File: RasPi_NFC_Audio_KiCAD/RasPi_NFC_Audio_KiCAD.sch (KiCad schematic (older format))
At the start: 21 parts, among them J1 Barrel_Jack_Switch, J2 Conn_02x20_Odd_Even, J3 Connector_01x10, U1 MIC5225-3.3V

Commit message: Layout updates
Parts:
- J2: footprint Connector_PinSocket_2.54mm:PinSocket_2x20_P2.54mm_Vertical -> Connector_PinHeader_2.54mm:PinHeader_2x20_P2.54mm_Vertical
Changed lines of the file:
@@
 EESchema Schematic File Version 4
 LIBS:RasPi_NFC_Audio_KiCAD-cache
-EELAYER 30 0
+EELAYER 29 0
 EELAYER END
 $Descr A4 11693 8268
@@
 F 0 "J2" H 4130 6450 50  0000 C CNN
 F 1 "Conn_02x20_Odd_Even" H 4140 6416 50  0001 C CNN
-F 2 "Connector_PinSocket_2.54mm:PinSocket_2x20_P2.54mm_Vertical" H -760 4440 50  0001 C CNN
+F 2 "Connector_PinHeader_2.54mm:PinHeader_2x20_P2.54mm_Vertical" H -760 4440 50  0001 C CNN
 F 3 "" H -760 4440 50  0001 C CNN
 F 4 "M20-7831046" H 4090 5390 50  0001 C CNN "Part #"

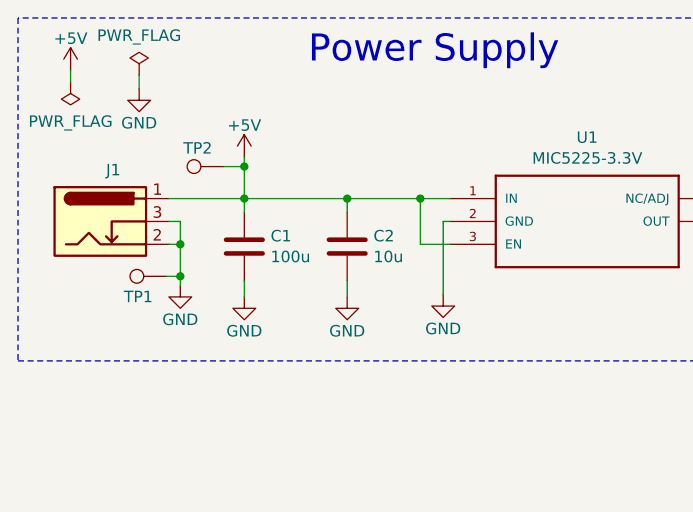
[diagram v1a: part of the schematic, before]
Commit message: Layout updates
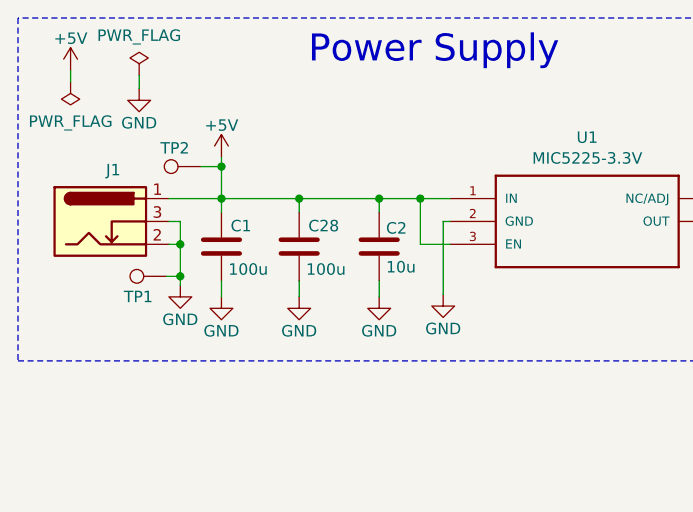
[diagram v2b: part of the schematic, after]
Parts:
- added C28: 100u, Capacitor_SMD:C_1206_3216Metric_Pad1.42x1.75mm_HandSolder, symbol Device:C
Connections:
- net +5V: now also C28.1
- net GND: now also C28.2
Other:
- moved on the sheet: C1, C2, TP2
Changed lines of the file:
@@
 EESchema Schematic File Version 4
 LIBS:RasPi_NFC_Audio_KiCAD-cache
-EELAYER 29 0
+EELAYER 30 0
 EELAYER END
 $Descr A4 11693 8268
@@
 L Device:C C1
 U 1 1 5E1A86EE
-P 2060 2330
-F 0 "C1" H 2175 2376 50  0000 L CNN
-F 1 "100u" H 2175 2285 50  0000 L CNN
-F 2 "Capacitor_SMD:C_1206_3216Metric_Pad1.42x1.75mm_HandSolder" H 2098 2180 50  0001 C CNN
-F 3 "~" H 2060 2330 50  0001 C CNN
-F 4 "GRM31CD80J107ME39L" H 2060 2330 50  0001 C CNN "Part #"
-F 5 "490-10525-1-ND" H 2060 2330 50  0001 C CNN "DigiKey"
-	1    2060 2330
+P 1960 2330
+F 0 "C1" H 2000 2420 50  0000 L CNN
+F 1 "100u" H 1990 2230 50  0000 L CNN
+F 2 "Capacitor_SMD:C_1206_3216Metric_Pad1.42x1.75mm_HandSolder" H 1998 2180 50  0001 C CNN
+F 3 "~" H 1960 2330 50  0001 C CNN
+F 4 "GRM31CD80J107ME39L" H 1960 2330 50  0001 C CNN "Part #"
+F 5 "490-10525-1-ND" H 1960 2330 50  0001 C CNN "DigiKey"
+	1    1960 2330
 	1    0    0    -1
 $EndComp
@@
 L Device:C C2
 U 1 1 5E1AABBB
-P 2510 2330
-F 0 "C2" H 2625 2376 50  0000 L CNN
-F 1 "10u" H 2625 2285 50  0000 L CNN
-F 2 "Capacitor_SMD:C_0603_1608Metric_Pad1.05x0.95mm_HandSolder" H 2548 2180 50  0001 C CNN
-F 3 "~" H 2510 2330 50  0001 C CNN
-F 4 "CL10A106MQ8NNNC" H 2510 2330 50  0001 C CNN "Part #"
-F 5 "1276-1119-1-ND" H 2510 2330 50  0001 C CNN "DigiKey"
-	1    2510 2330
+P 2650 2330
+F 0 "C2" H 2680 2410 50  0000 L CNN
+F 1 "10u" H 2680 2240 50  0000 L CNN
+F 2 "Capacitor_SMD:C_0603_1608Metric_Pad1.05x0.95mm_HandSolder" H 2688 2180 50  0001 C CNN
+F 3 "~" H 2650 2330 50  0001 C CNN
+F 4 "CL10A106MQ8NNNC" H 2650 2330 50  0001 C CNN "Part #"
+F 5 "1276-1119-1-ND" H 2650 2330 50  0001 C CNN "DigiKey"
+	1    2650 2330
 	1    0    0    -1
 $EndComp
@@
 L power:GND #PWR0102
 U 1 1 5E1B33E8
-P 2060 2550
-F 0 "#PWR0102" H 2060 2300 50  0001 C CNN
-F 1 "GND" H 2060 2400 50  0000 C CNN
-F 2 "" H 2060 2550 50  0000 C CNN
-F 3 "" H 2060 2550 50  0000 C CNN
-	1    2060 2550
+P 1960 2550
+F 0 "#PWR0102" H 1960 2300 50  0001 C CNN
+F 1 "GND" H 1960 2400 50  0000 C CNN
+F 2 "" H 1960 2550 50  0000 C CNN
+F 3 "" H 1960 2550 50  0000 C CNN
+	1    1960 2550
 	1    0    0    -1
 $EndComp
@@
 L power:GND #PWR0103
 U 1 1 5E1B3827
-P 2510 2550
-F 0 "#PWR0103" H 2510 2300 50  0001 C CNN
-F 1 "GND" H 2510 2400 50  0000 C CNN
-F 2 "" H 2510 2550 50  0000 C CNN
-F 3 "" H 2510 2550 50  0000 C CNN
-	1    2510 2550
-	1    0    0    -1
-$EndComp
-Wire Wire Line
-	2060 2550 2060 2480
-Wire Wire Line
-	2510 2550 2510 2480
-Wire Wire Line
-	2060 2180 2060 2120
-Wire Wire Line
-	2510 2180 2510 2120
+P 2650 2550
+F 0 "#PWR0103" H 2650 2300 50  0001 C CNN
+F 1 "GND" H 2650 2400 50  0000 C CNN
+F 2 "" H 2650 2550 50  0000 C CNN
+F 3 "" H 2650 2550 50  0000 C CNN
+	1    2650 2550
+	1    0    0    -1
+$EndComp
+Wire Wire Line
+	1960 2550 1960 2480
+Wire Wire Line
+	2650 2550 2650 2480
+Wire Wire Line
+	2650 2180 2650 2120
 $Comp
 L power:GND #PWR0104
@@
 Wire Wire Line
 	2830 2120 2960 2120
-Connection ~ 2060 2120
-Wire Wire Line
-	2060 2120 2510 2120
-Connection ~ 2510 2120
-Wire Wire Line
-	2510 2120 2830 2120
+Connection ~ 2650 2120
 $Comp
 L power:+5V #PWR0106
 U 1 1 5E1C9964
-P 2060 1940
-F 0 "#PWR0106" H 2060 1790 50  0001 C CNN
-F 1 "+5V" H 2060 2080 50  0000 C CNN
-F 2 "" H 2060 1940 50  0000 C CNN
-F 3 "" H 2060 1940 50  0000 C CNN
-	1    2060 1940
+P 1960 1940
+F 0 "#PWR0106" H 1960 1790 50  0001 C CNN
+F 1 "+5V" H 1960 2080 50  0000 C CNN
+F 2 "" H 1960 1940 50  0000 C CNN
+F 3 "" H 1960 1940 50  0000 C CNN
+	1    1960 1940
 	1    0    0    -1
 $EndComp
@@
 $EndComp
 Wire Wire Line
-	2060 1940 2060 1980
+	1960 1940 1960 1980
 $Comp
 L power:VCOM #PWR0108
@@
 L Connector:TestPoint TP2
 U 1 1 5E2FD82C
-P 1970 1980
-F 0 "TP2" V 2050 2030 50  0000 L CNN
-F 1 "TestPoint" H 2028 2007 50  0001 L CNN
-F 2 "TestPoint:TestPoint_Keystone_5019_Minature" H 2170 1980 50  0001 C CNN
-F 3 "~" H 2170 1980 50  0001 C CNN
-	1    1970 1980
+P 1870 1980
+F 0 "TP2" V 1950 2030 50  0000 L CNN
+F 1 "TestPoint" H 1928 2007 50  0001 L CNN
+F 2 "TestPoint:TestPoint_Keystone_5019_Minature" H 2070 1980 50  0001 C CNN
+F 3 "~" H 2070 1980 50  0001 C CNN
+	1    1870 1980
 	0    -1   -1   0
 $EndComp
 Wire Wire Line
-	1730 2120 2060 2120
-Wire Wire Line
-	1970 1980 2060 1980
-Connection ~ 2060 1980
-Wire Wire Line
-	2060 1980 2060 2120
+	1730 2120 1960 2120
+Wire Wire Line
+	1870 1980 1960 1980
+Connection ~ 1960 1980
+Wire Wire Line
+	1960 1980 1960 2120
 $Comp
 L Connector:TestPoint TP1
@@
 Wire Wire Line
 	1600 1580 1600 1640
+Connection ~ 1960 2120
+Wire Wire Line
+	1960 2180 1960 2120
+Wire Wire Line
+	2650 2120 2830 2120
+Wire Wire Line
+	1960 2120 2300 2120
+$Comp
+L Device:C C28
+U 1 1 5E23A078
+P 2300 2330
+F 0 "C28" H 2340 2420 50  0000 L CNN
+F 1 "100u" H 2330 2230 50  0000 L CNN
+F 2 "Capacitor_SMD:C_1206_3216Metric_Pad1.42x1.75mm_HandSolder" H 2338 2180 50  0001 C CNN
+F 3 "~" H 2300 2330 50  0001 C CNN
+F 4 "GRM31CD80J107ME39L" H 2300 2330 50  0001 C CNN "Part #"
+F 5 "490-10525-1-ND" H 2300 2330 50  0001 C CNN "DigiKey"
+	1    2300 2330
+	1    0    0    -1
+$EndComp
+$Comp
+L power:GND #PWR06
+U 1 1 5E23A7C7
+P 2300 2550
+F 0 "#PWR06" H 2300 2300 50  0001 C CNN
+F 1 "GND" H 2300 2400 50  0000 C CNN
+F 2 "" H 2300 2550 50  0000 C CNN
+F 3 "" H 2300 2550 50  0000 C CNN
+	1    2300 2550
+	1    0    0    -1
+$EndComp
+Wire Wire Line
+	2300 2550 2300 2480
+Wire Wire Line
+	2300 2180 2300 2120
+Connection ~ 2300 2120
+Wire Wire Line
+	2300 2120 2650 2120
 $EndSCHEMATC

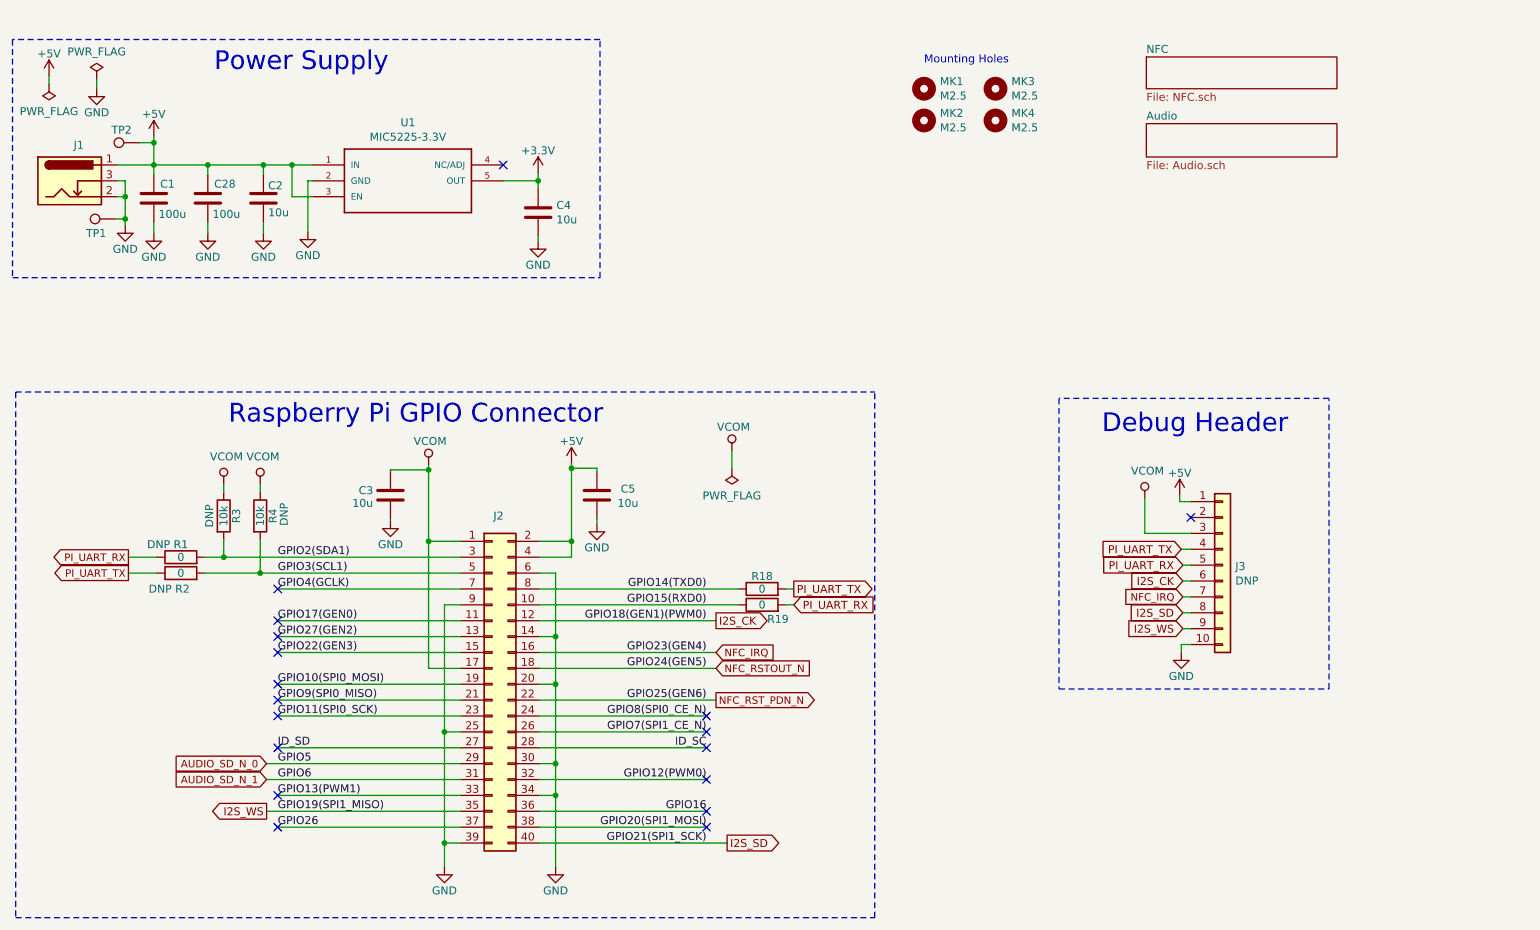
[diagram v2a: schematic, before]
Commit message: Layout updates
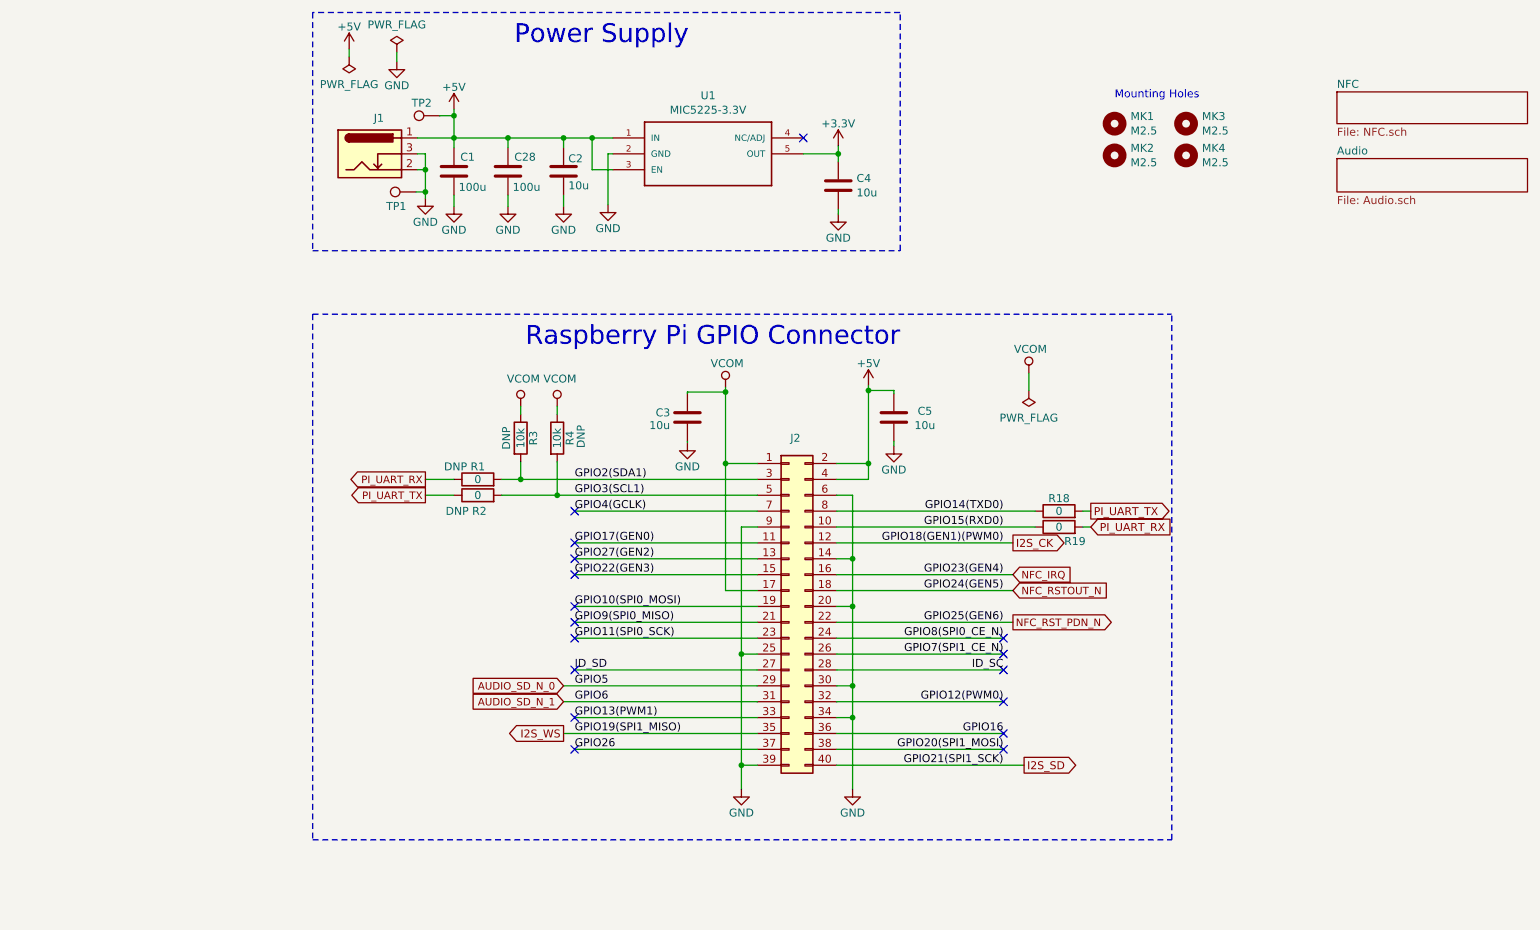
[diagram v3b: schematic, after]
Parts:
- removed J3: Connector_01x10, Connector_PinHeader_2.54mm:PinHeader_1x10_P2.54mm_Vertical, symbol Connector_Generic:Conn_01x10
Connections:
- no-connect marks 18 -> 17
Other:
- note removed: "Debug Header"
- moved on the sheet: C1, C2, C28, C3, C4, C5, J1, J2, MK1, MK2, MK3, MK4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
